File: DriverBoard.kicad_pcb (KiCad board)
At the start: 2 copper layers, 80 x 60 mm, 104 parts, among them J1 Conn_02x07_Odd_Even, J2 Conn_02x07_Odd_Even, Q1 HYG025N06LS1C2, Q2 HYG025N06LS1C2, Q3 HYG025N06LS1C2, Q4 HYG025N06LS1C2, Q5 HYG025N06LS1C2, Q6 HYG025N06LS1C2, U2 SCT2420, U3 SCT2610

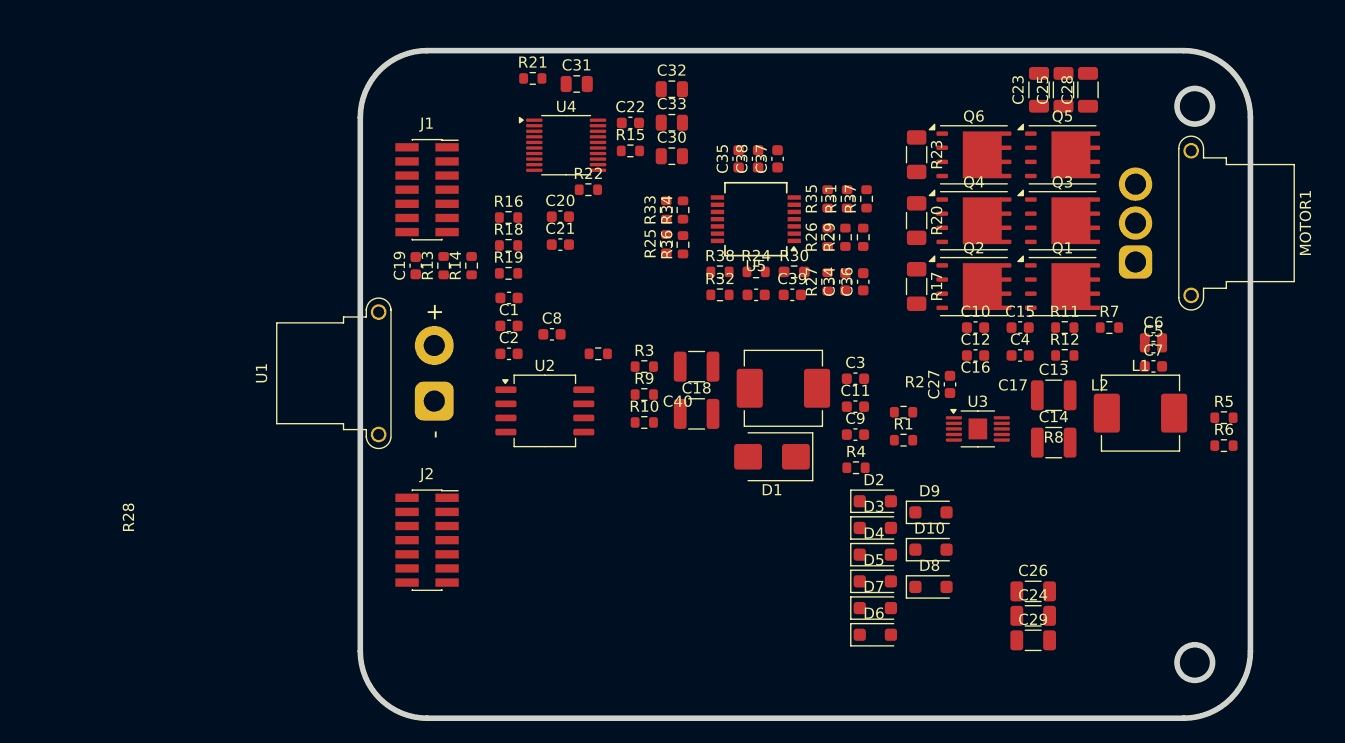
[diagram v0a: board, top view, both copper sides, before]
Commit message: 修改板框文件
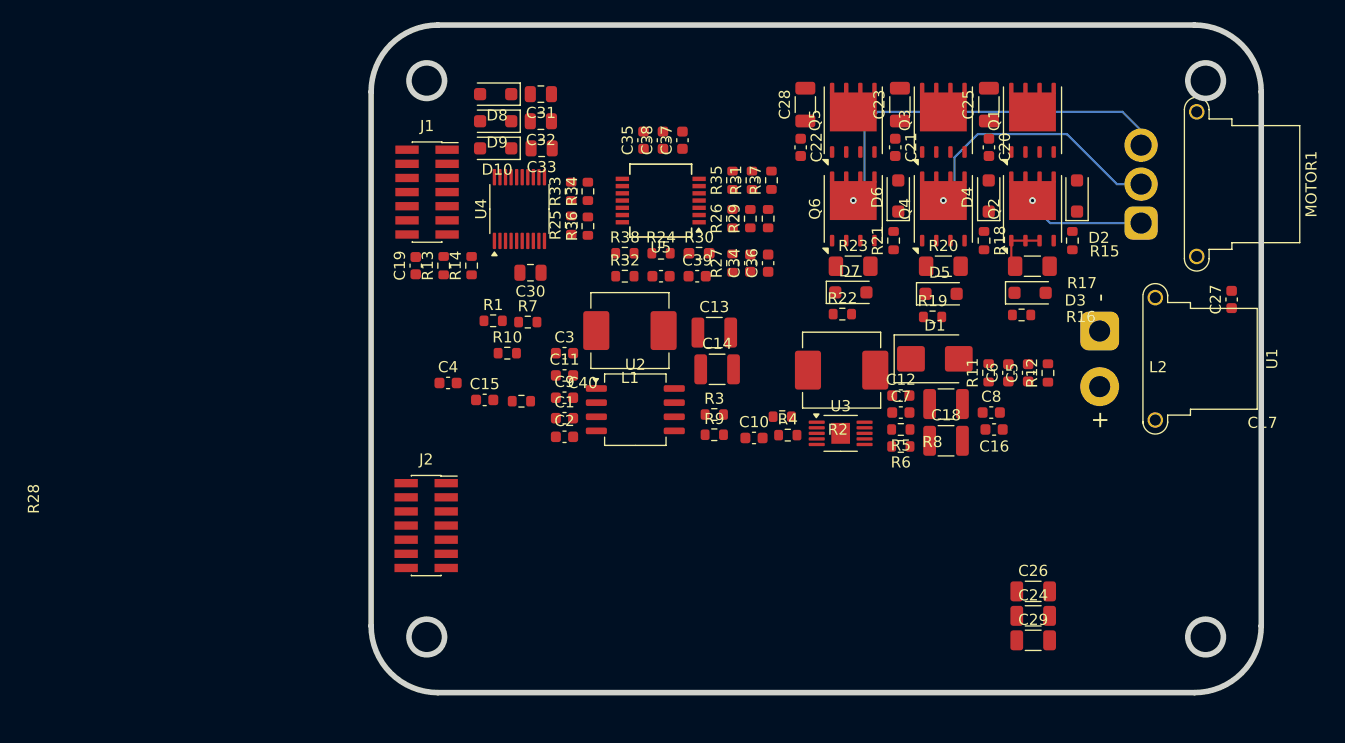
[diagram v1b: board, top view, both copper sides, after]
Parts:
- moved U1 60.1 mm to (182.4, 73.7), turned to -90 degrees
- moved D8 59.1 mm to (128.2, 52.4), turned to 180 degrees
- moved D10 53.2 mm to (128.2, 57.3), turned to 180 degrees
- moved D9 52.6 mm to (128.2, 54.8), turned to 180 degrees
- moved R7 52.3 mm to (131.1, 72.9)
- moved C4 51.5 mm to (123.9, 78.4)
- moved C15 48.6 mm to (127.2, 79.9)
- moved R16 46.9 mm to (175.4, 72.3)
- moved L1 46.5 mm to (140.2, 73.7), turned to 180 degrees
- moved C16 45.2 mm to (173.0, 82.5)
- moved R18 42.7 mm to (172.1, 65.6), turned to -90 degrees
- moved R15 40.5 mm to (180.0, 65.6), turned to 90 degrees
- moved C8 40.1 mm to (172.7, 81.0)
- moved D6 39.5 mm to (164.3, 61.6), turned to 90 degrees
- moved C20 39.0 mm to (172.5, 57.2), turned to -90 degrees
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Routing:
- net /Pre_Driver/W1: track 0.00 -> 33.8 mm, vias 0 -> 1
- net /Pre_Driver/V1: track 0.00 -> 23.0 mm, vias 0 -> 1
- net /Pre_Driver/U1: track 0.00 -> 10.8 mm, vias 0 -> 1
- net /ThreePhase/U1_CURR: track 0.00 -> 4.98 mm
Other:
- outline, holes or cut-outs redrawn
